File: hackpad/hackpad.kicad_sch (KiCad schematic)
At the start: 7 parts, among them SW1 SW_Push, SW2 SW_Push, SW3 SW_Push, SW4 SW_Push, U1 XIAO-RP2040-DIP

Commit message: pcb v1 done
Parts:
- U1: footprint Module:MOUDLE14P-XIAO-DIP-SMD -> Seeed Studio XIAO Series Library:XIAO-RP2040-DIP
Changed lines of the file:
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@@
 			)
 		)
-		(property "Footprint" "Module:MOUDLE14P-XIAO-DIP-SMD"
+		(property "Footprint" "Seeed Studio XIAO Series Library:XIAO-RP2040-DIP"
 			(at 192.278 132.588 0)
 			(effects

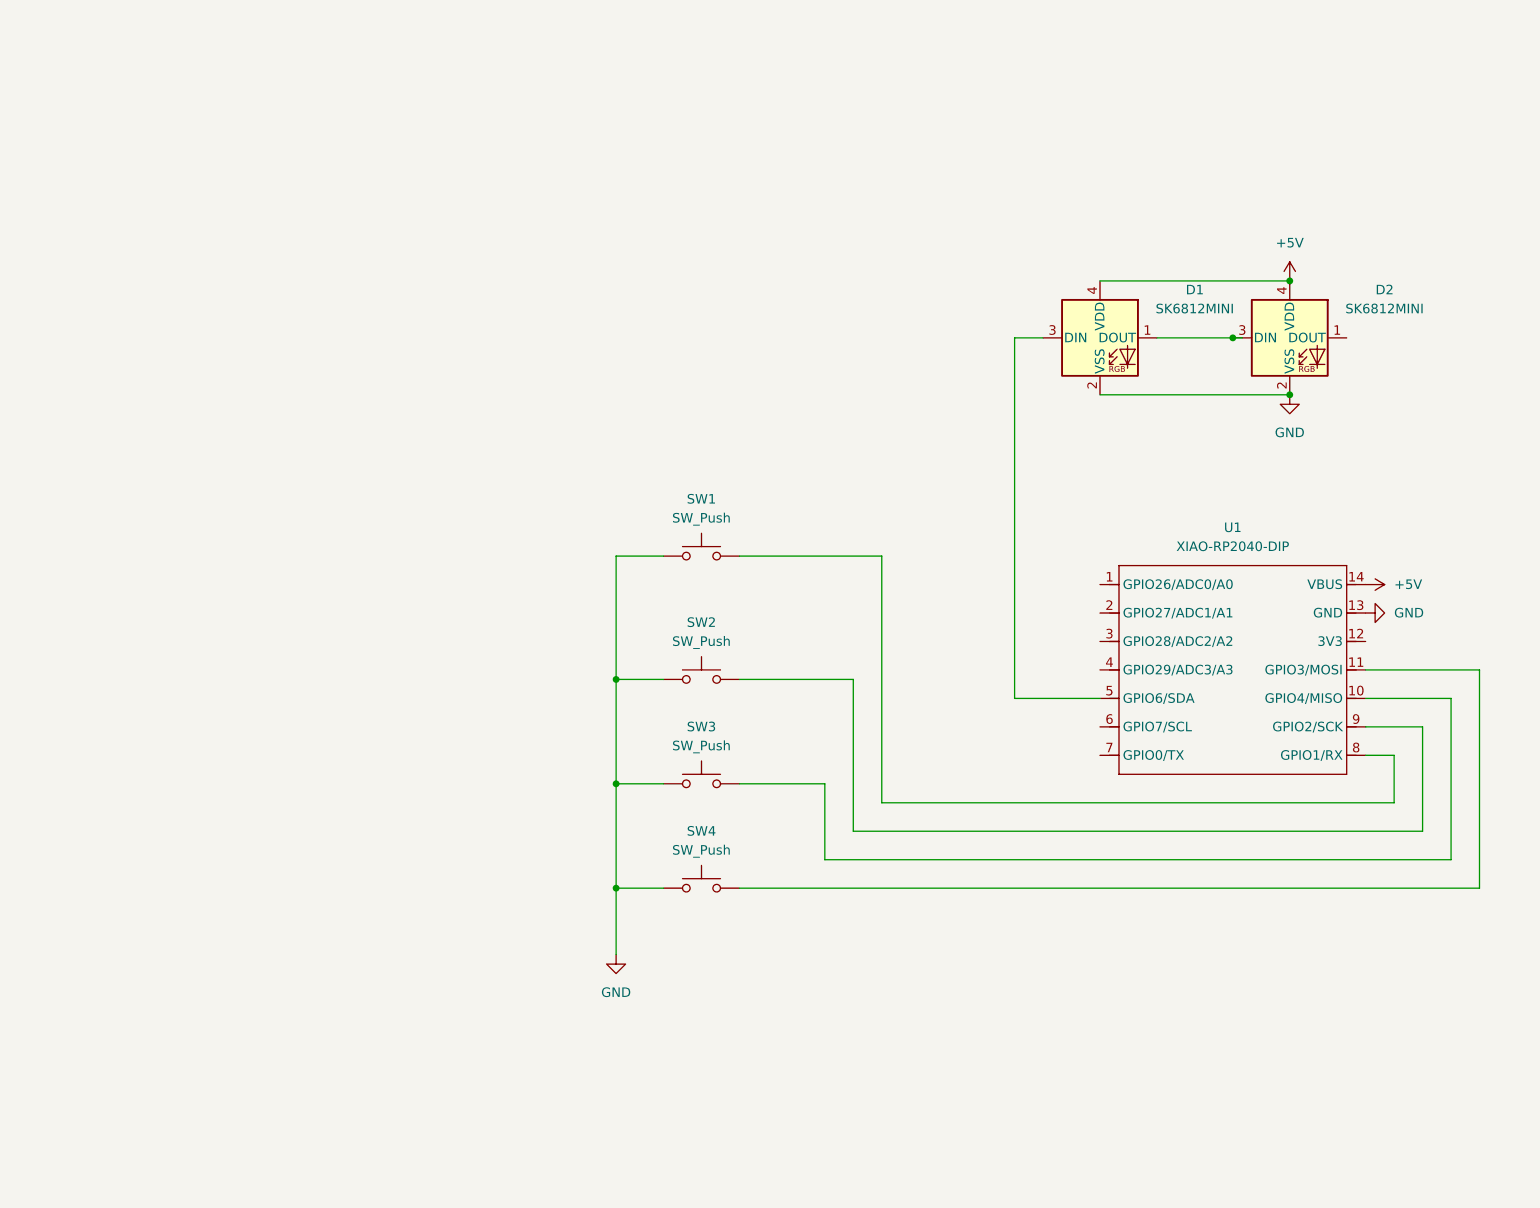
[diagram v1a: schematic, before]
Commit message: v2 done?
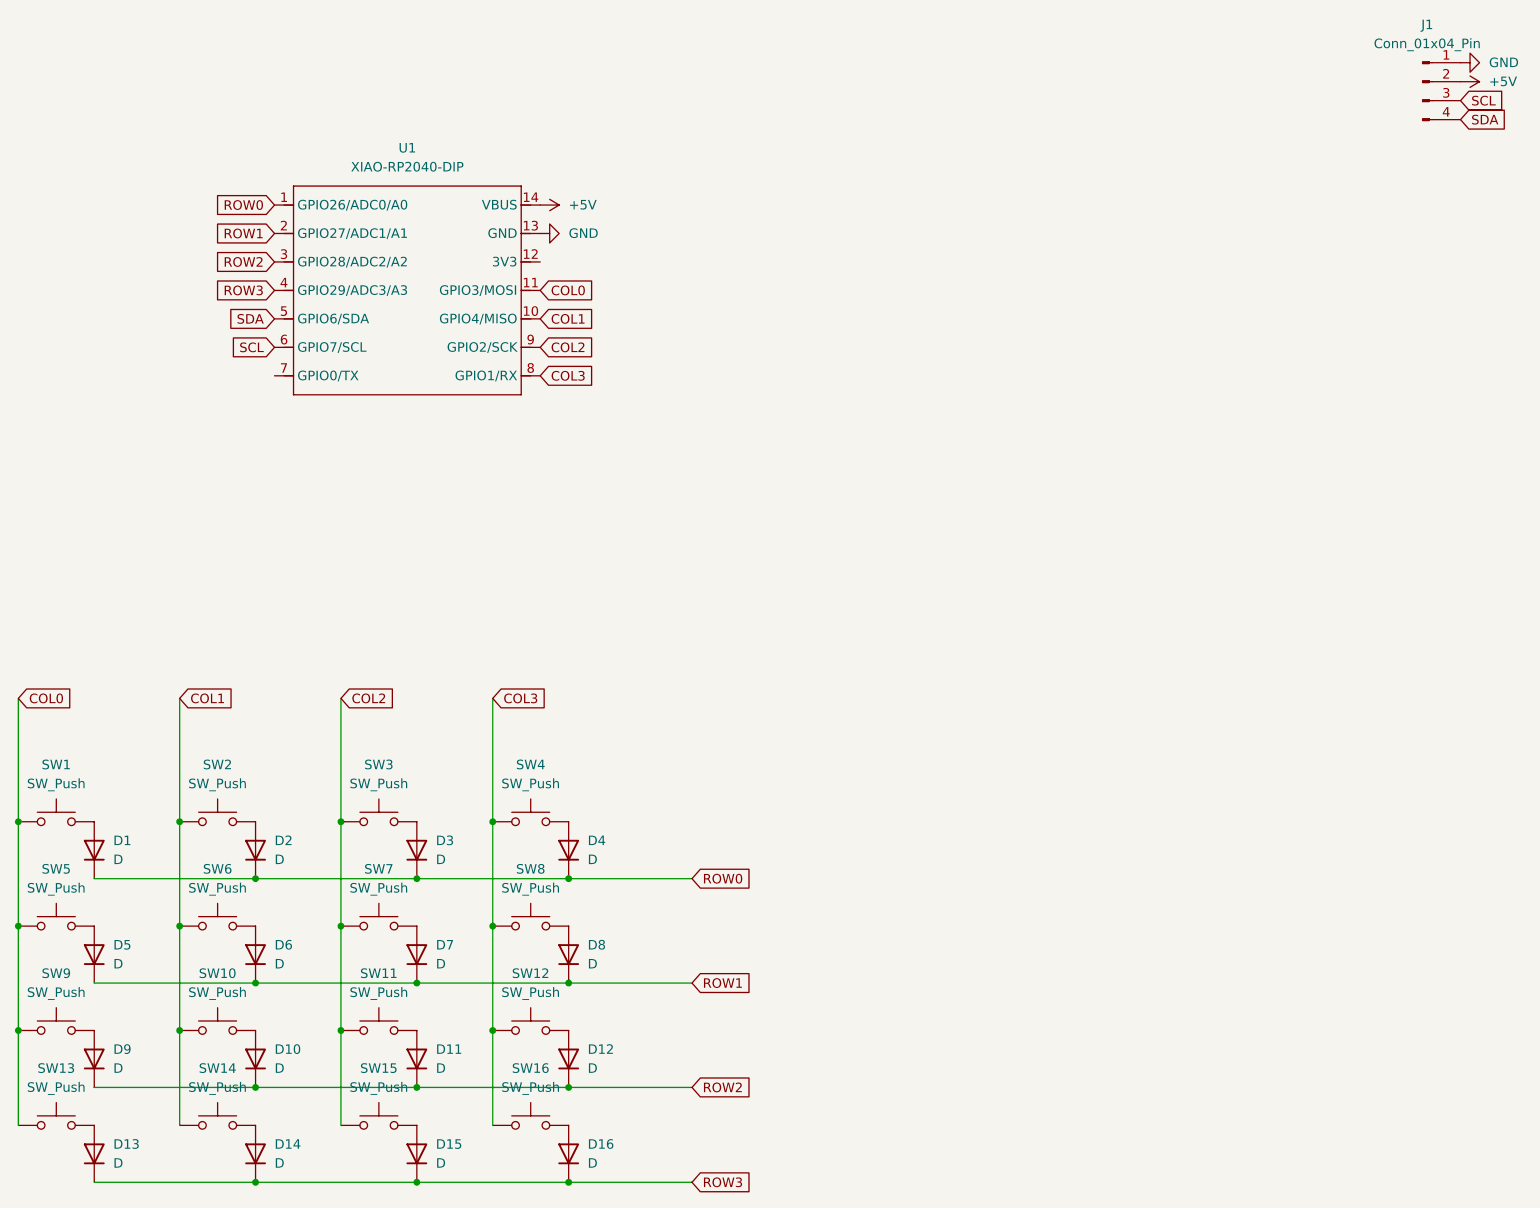
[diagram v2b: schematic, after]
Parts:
- removed D1, D2: SK6812MINI, LED_SMD:LED_SK6812MINI_PLCC4_3.5x3.5mm_P1.75mm, symbol LED:SK6812MINI
- added D1, D10, D11, D12, D13, D14, D15, D16, D2, D3, D4, D5, D6, D7, D8, D9: D, Diode_THT:D_DO-35_SOD27_P7.62mm_Horizontal, symbol Device:D
- added J1: Conn_01x04_Pin, OLED:SSD1306-0.91-OLED-4pin-128x32, symbol Connector:Conn_01x04_Pin
- added SW10, SW11, SW12, SW13, SW14, SW15, SW16, SW5, SW6, SW7, SW8, SW9: SW_Push, Button_Switch_Keyboard:SW_Cherry_MX_1.00u_PCB, symbol Switch:SW_Push
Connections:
- net +5V: now also J1.2 (Pin_2)
- net GND: now also J1.1 (Pin_1); no longer SW1.1, SW2.1, SW3.1, SW4.1
- net at SW3.2: now also D3.2 (A); no longer U1.10 (GPIO4/MISO)
- net ROW0: now reaches U1.1 (GPIO26/ADC0/A0)
- net ROW0: now also D1.1 (K), D2.1 (K), D3.1 (K), D4.1 (K)
- net at SW4.2: now also D4.2 (A); no longer U1.11 (GPIO3/MOSI)
- net ROW1: now reaches U1.2 (GPIO27/ADC1/A1)
- net ROW1: now also D5.1 (K), D6.1 (K), D7.1 (K), D8.1 (K)
- net ROW2: now reaches U1.3 (GPIO28/ADC2/A2)
- net ROW2: now also D10.1 (K), D11.1 (K), D12.1 (K), D9.1 (K)
- net ROW3: now reaches U1.4 (GPIO29/ADC3/A3)
- net ROW3: now also D13.1 (K), D14.1 (K), D15.1 (K), D16.1 (K)
- net SDA: now reaches U1.5 (GPIO6/SDA)
- net SDA: now also J1.4 (Pin_4)
- net SCL: now reaches U1.6 (GPIO7/SCL)
- net SCL: now also J1.3 (Pin_3)
- net at SW1.2: now also D1.2 (A); no longer U1.8 (GPIO1/RX)
- net at SW2.2: now also D2.2 (A); no longer U1.9 (GPIO2/SCK)
- new net: D14.2 (A), SW14.2
- new net: D15.2 (A), SW15.2
- new net: D9.2 (A), SW9.2
- new net: D6.2 (A), SW6.2
- new net: D7.2 (A), SW7.2
- new net: D5.2 (A), SW5.2
- new net: D8.2 (A), SW8.2
- new net: D13.2 (A), SW13.2
- new net: D16.2 (A), SW16.2
- new net: D10.2 (A), SW10.2
- new net: D11.2 (A), SW11.2
- new net: D12.2 (A), SW12.2
- new net COL0: SW1.1, SW13.1, SW5.1, SW9.1, U1.11 (GPIO3/MOSI)
- new net COL1: SW10.1, SW14.1, SW2.1, SW6.1, U1.10 (GPIO4/MISO)
- new net COL2: SW11.1, SW15.1, SW3.1, SW7.1, U1.9 (GPIO2/SCK)
- new net COL3: SW12.1, SW16.1, SW4.1, SW8.1, U1.8 (GPIO1/RX)
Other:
- moved on the sheet: U1
